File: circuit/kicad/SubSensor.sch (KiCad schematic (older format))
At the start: 5 parts, among them J1 SH3, U1 S7136

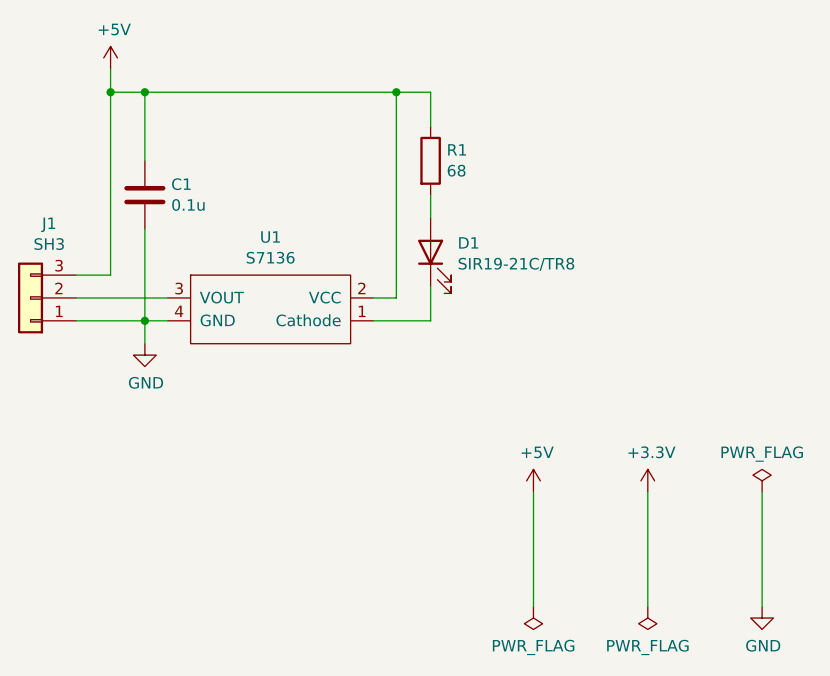
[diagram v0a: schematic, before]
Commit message: hoge
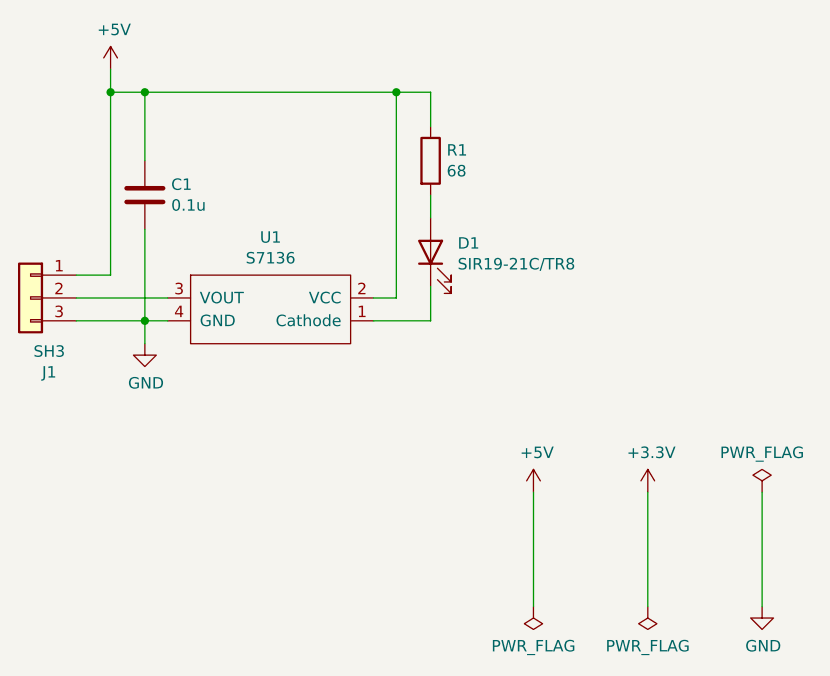
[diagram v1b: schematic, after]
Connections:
- net +5V: now also J1.1 (Pin_1); no longer J1.3 (Pin_3)
- net GND: now also J1.3 (Pin_3); no longer J1.1 (Pin_1)
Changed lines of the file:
@@
 $Descr A4 11693 8268
 encoding utf-8
-Sheet 5 5
+Sheet 1 1
 Title ""
 Date ""
@@
 F 3 "~" H 3050 4450 50  0001 C CNN
 	1    3050 4450
-	-1   0    0    1
+	-1   0    0    -1
 $EndComp
 Wire Wire Line
